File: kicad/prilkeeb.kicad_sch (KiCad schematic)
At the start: 75 parts, among them SW1 SW_SPDT, U2 Nice_Nano_V2

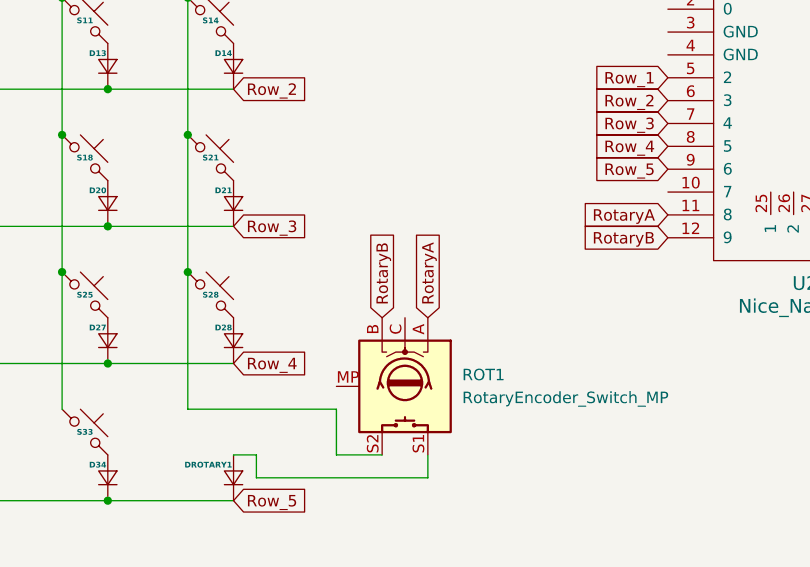
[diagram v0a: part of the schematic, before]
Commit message: Routing
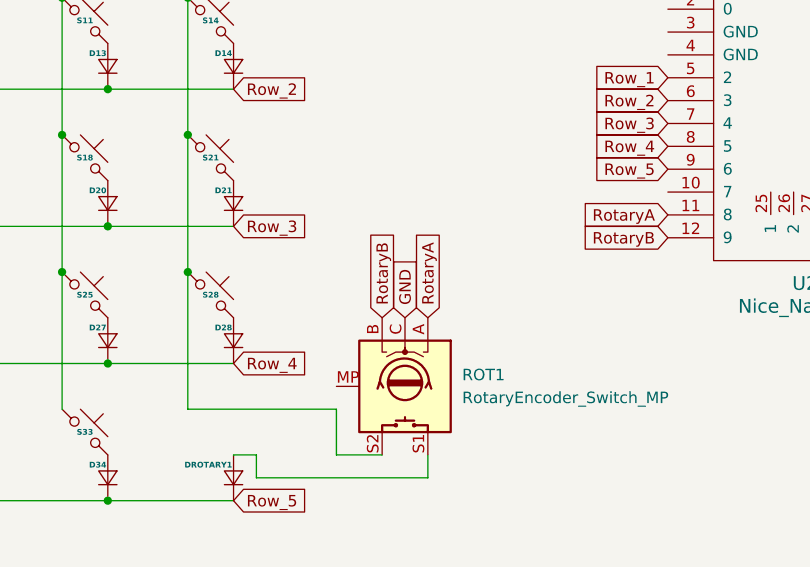
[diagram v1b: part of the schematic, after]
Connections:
- net GND: now also ROT1.C
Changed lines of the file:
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@@
+		)
+	)
+	(global_label "GND"
+		(shape input)
+		(at 147.32 121.92 90)
+		(fields_autoplaced yes)
+		(effects
+			(font
+				(size 1.27 1.27)
+			)
+			(justify left)
+		)
+		(property "Intersheetrefs" "${INTERSHEET_REFS}"
+			(at 147.32 115.0643 90)
+			(effects
+				(font
+					(size 1.27 1.27)
+				)
+				(justify left)
+				(hide yes)
+			)
 		)
 	)
